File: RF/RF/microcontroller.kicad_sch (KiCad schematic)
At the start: 21 parts, among them IC201 CC1110F16RHHR

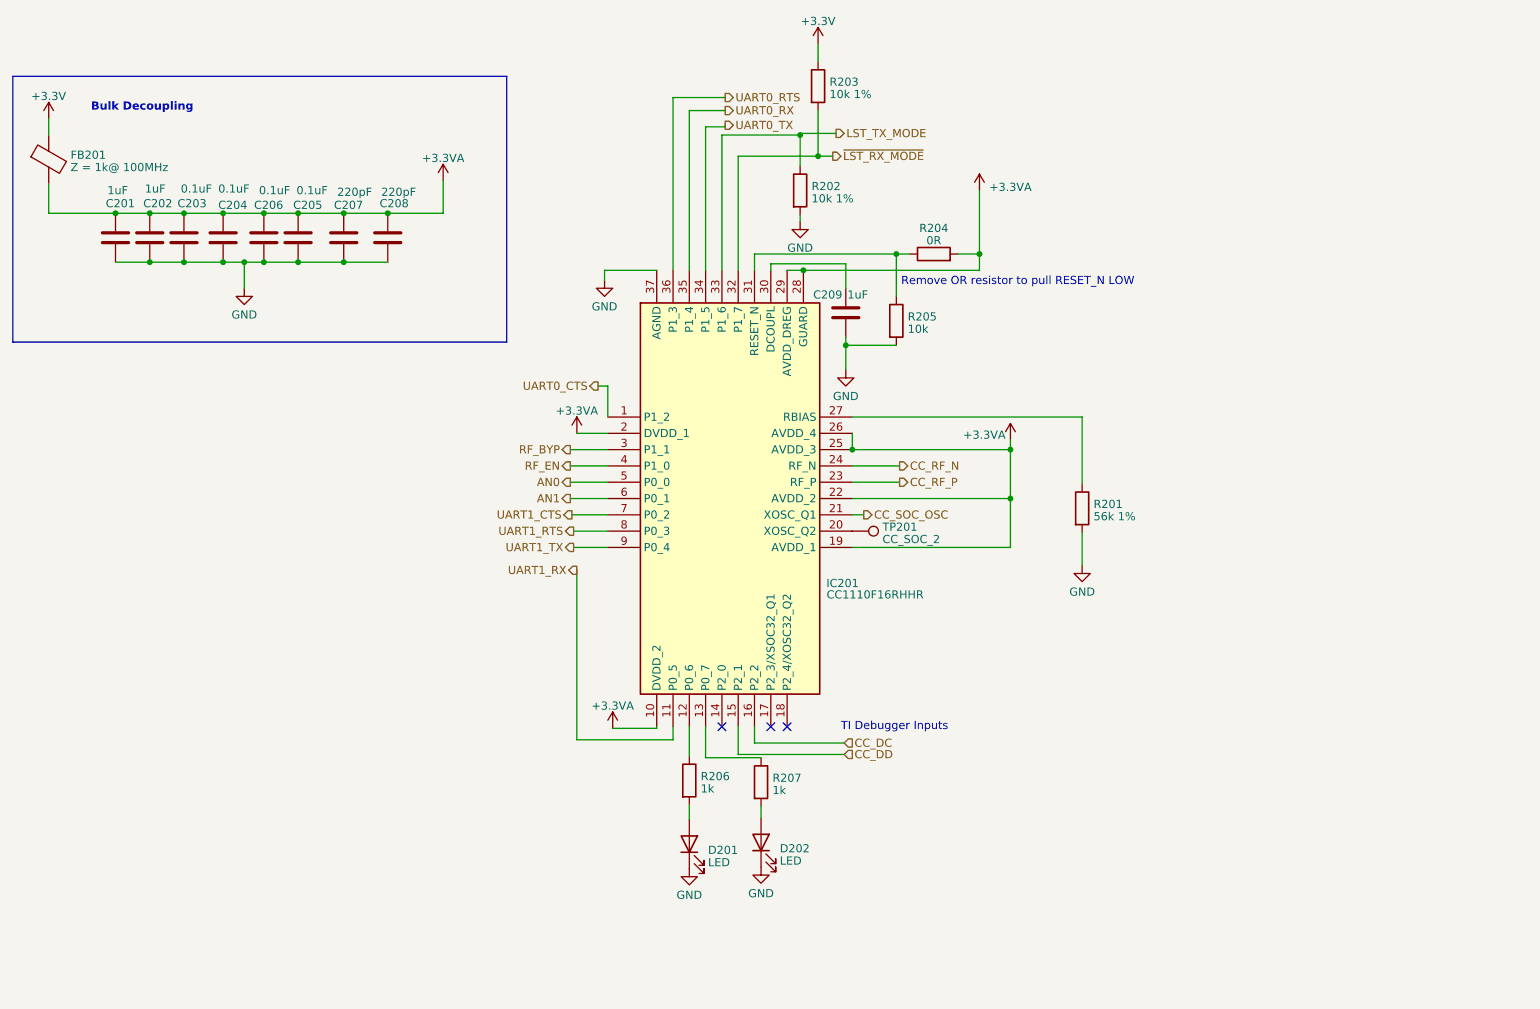
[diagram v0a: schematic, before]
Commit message: added external memory
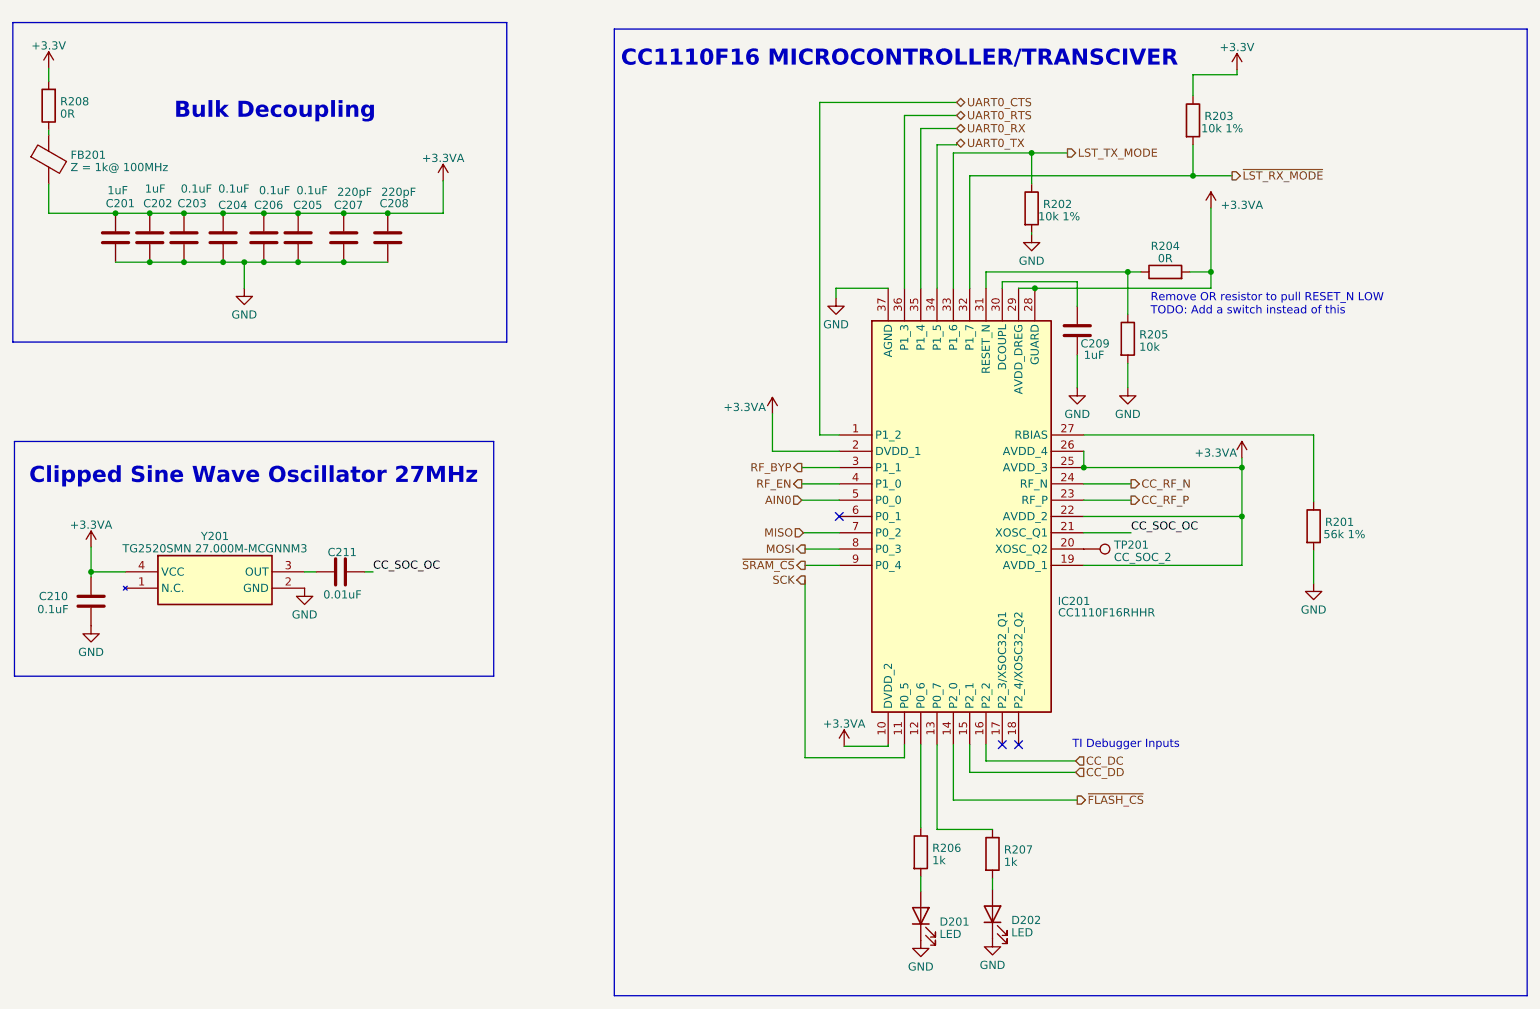
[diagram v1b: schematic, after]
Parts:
- added C210: 0.1uF, Capacitor_SMD:C_0603_1608Metric_Pad1.08x0.95mm_HandSolder, symbol Device:C
- added C211: 0.01uF, Capacitor_SMD:C_0603_1608Metric_Pad1.08x0.95mm_HandSolder, symbol Device:C
- added R208: 0R, Resistor_SMD:R_0603_1608Metric_Pad0.98x0.95mm_HandSolder, symbol Device:R
- added Y201: TG2520SMN 27.000M-MCGNNM3, SamacSys_Parts:TG2520SMN25000MMCGNNM3, symbol SamacSys_Parts:TG2520SMN_25.000M-MCGNNM3
- C201, C202, C203, C204, C205, C206, C207, C208, C209: footprint (none) -> Capacitor_SMD:C_0603_1608Metric_Pad1.08x0.95mm_HandSolder
- D201, D202: footprint (none) -> LED_SMD:LED_0603_1608Metric_Pad1.05x0.95mm_HandSolder
- FB201: footprint (none) -> Inductor_SMD:L_0603_1608Metric_Pad1.05x0.95mm_HandSolder
- IC201: footprint QFN50P600X600X100-37N-D -> SamacSys_Parts:QFN50P600X600X100-37N-D
- R201, R202, R203, R204, R205, R206, R207: footprint (none) -> Resistor_SMD:R_0603_1608Metric_Pad0.98x0.95mm_HandSolder
- TP201: footprint (none) -> TestPoint:TestPoint_Loop_D3.50mm_Drill1.4mm_Beaded
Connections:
- net +3.3V: now also R208.2; no longer FB201.1
- net +3.3VA: now also C210.1, Y201.4 (VCC)
- net GND: now also C210.2, Y201.2 (GND)
- net ~{FLASH_CS}: now reaches IC201.14 (P2_0)
- net AN0 renamed AIN0
- net AN1: no longer names the net of IC201.6 (P0_1)
- net CC_SOC_OSC renamed CC_SOC_OC
- net CC_SOC_OC: now also C211.2
- net UART1_CTS renamed MISO
- net UART1_RTS renamed MOSI
- net UART1_RX renamed SCK
- net UART1_TX renamed ~{SRAM_CS}
- new net: C211.1, Y201.3 (OUT)
- new net: FB201.1, R208.1
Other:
- note added: "CC1110F16 MICROCONTROLLER/TRANSCIVER"
- note added: "Clipped Sine Wave Oscillator 27MHz"
- note added: "Remove OR resistor to pull RESET_N LOW TODO: Add a switch instead of this"
- note removed: "Remove OR resistor to pull RESET_N LOW"
- moved on the sheet: C209, D201, D202, IC201, R201, R202, R203, R204, R205, R206, R207, TP201
